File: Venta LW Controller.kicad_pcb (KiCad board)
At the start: 2 copper layers, 56 x 99.2 mm, 26 parts, among them J1 Conn_01x04, J2 Conn_02x05_Odd_Even, Q1 BSS138, Q2 BSS138, SW1 RST, SW2 FLASH, U1 LM2674N-3.3, U2 ESP32-WROOM-32

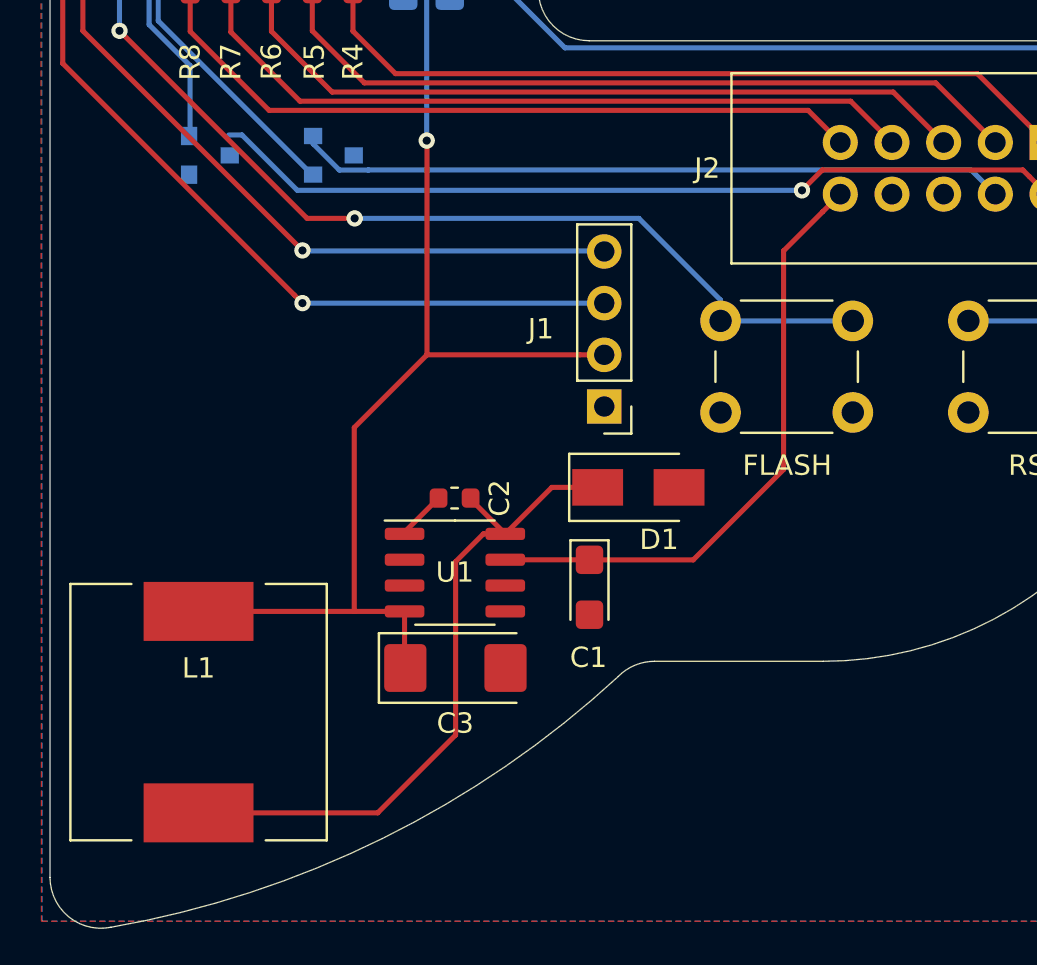
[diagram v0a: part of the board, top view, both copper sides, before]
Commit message: updated parts
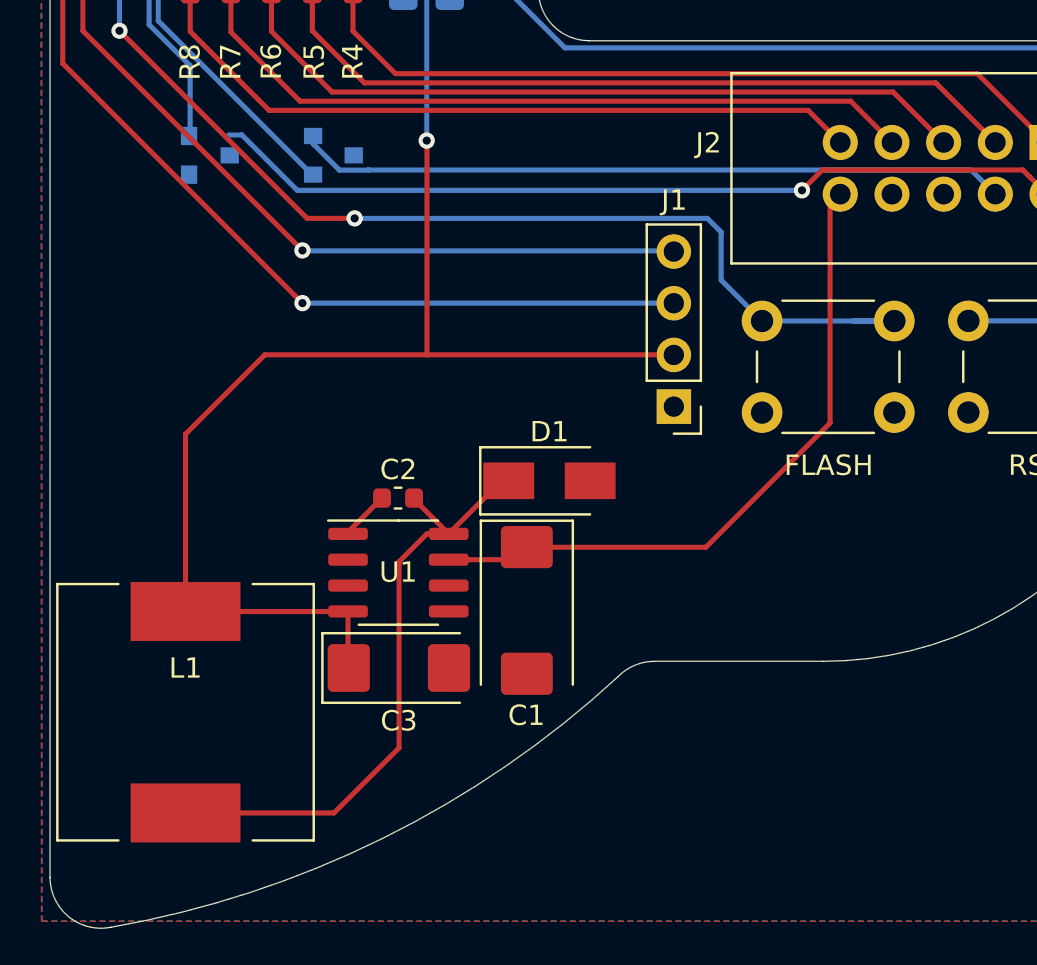
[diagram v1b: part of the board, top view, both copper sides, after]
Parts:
- C1: value 22u -> 22uF; footprint Capacitor_Tantalum_SMD:CP_EIA-3216-18_Kemet-A -> Capacitor_Tantalum_SMD:CP_EIA-7343-31_Kemet-D
- C2: value 0.01u -> 0.01uF
- C3: value 100u -> 100uF
- C4: value 10n -> 10nF
- C5: value 47u -> 47uF
- L1: value 100u -> 100uH
- R2, R4, R5, R6, R7, R8: value 10k -> 10K
- moved D1 4.38 mm to (149.0, 119.6)
- moved J1 3.42 mm to (155.2, 116.0)
- moved C1 3.28 mm to (147.9, 126.0)
- moved C2 2.78 mm to (141.6, 120.5)
- moved C3 2.78 mm to (141.6, 128.8)
- moved U1 2.78 mm to (141.6, 124.1)
- moved SW2 2.04 mm to (159.5, 111.8)
- moved L1 0.64 mm to (131.2, 131.0)
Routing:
- net +3.3V: track 80.9 -> 90.3 mm
- net FLASH: track 50.6 -> 55.5 mm
- net TXD: track 52.7 -> 56.1 mm
- net RXD: track 55.4 -> 58.8 mm
- net Net-(C2-Pad2): track 33.7 -> 30.5 mm
- net +24V: track 30.2 -> 33.0 mm
